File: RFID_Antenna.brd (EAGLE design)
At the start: 25.4 x 43.2 mm, 25 parts, among them J1 U.FL

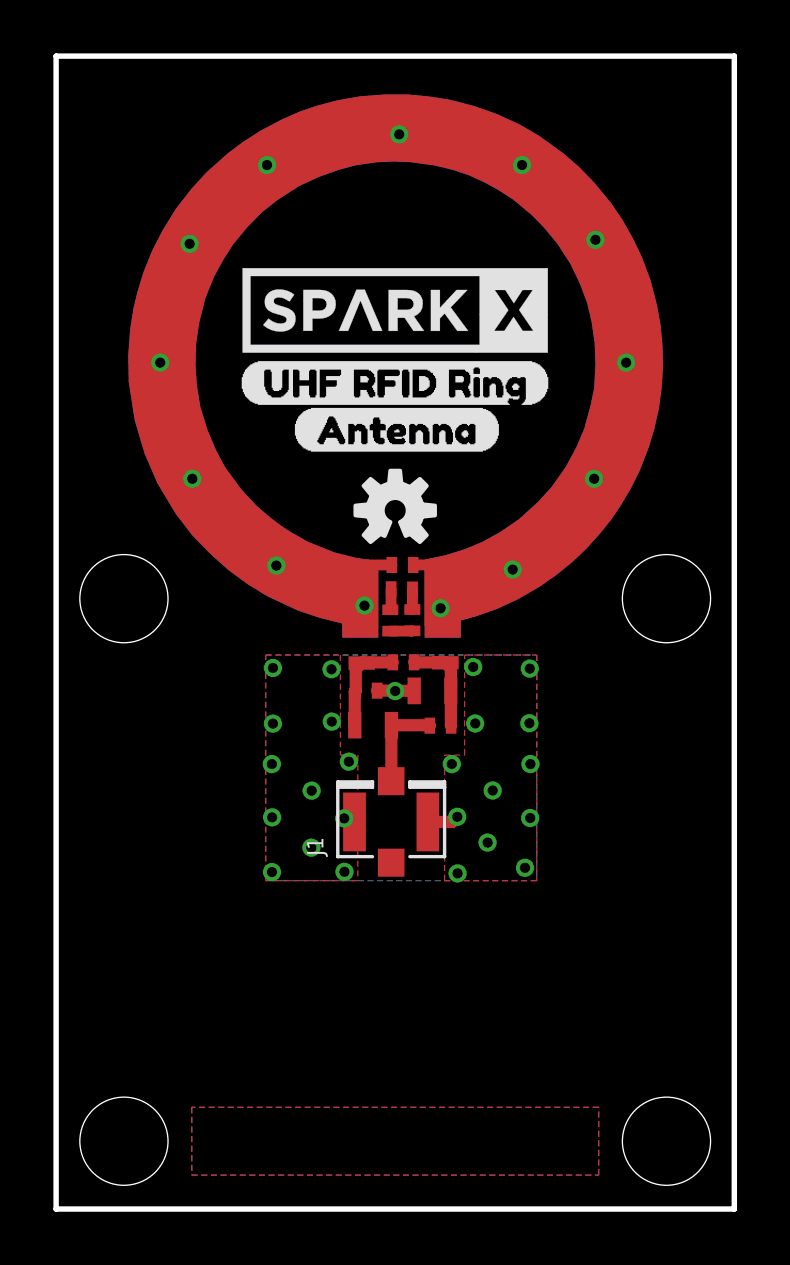
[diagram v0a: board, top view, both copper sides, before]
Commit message: Add production for x02
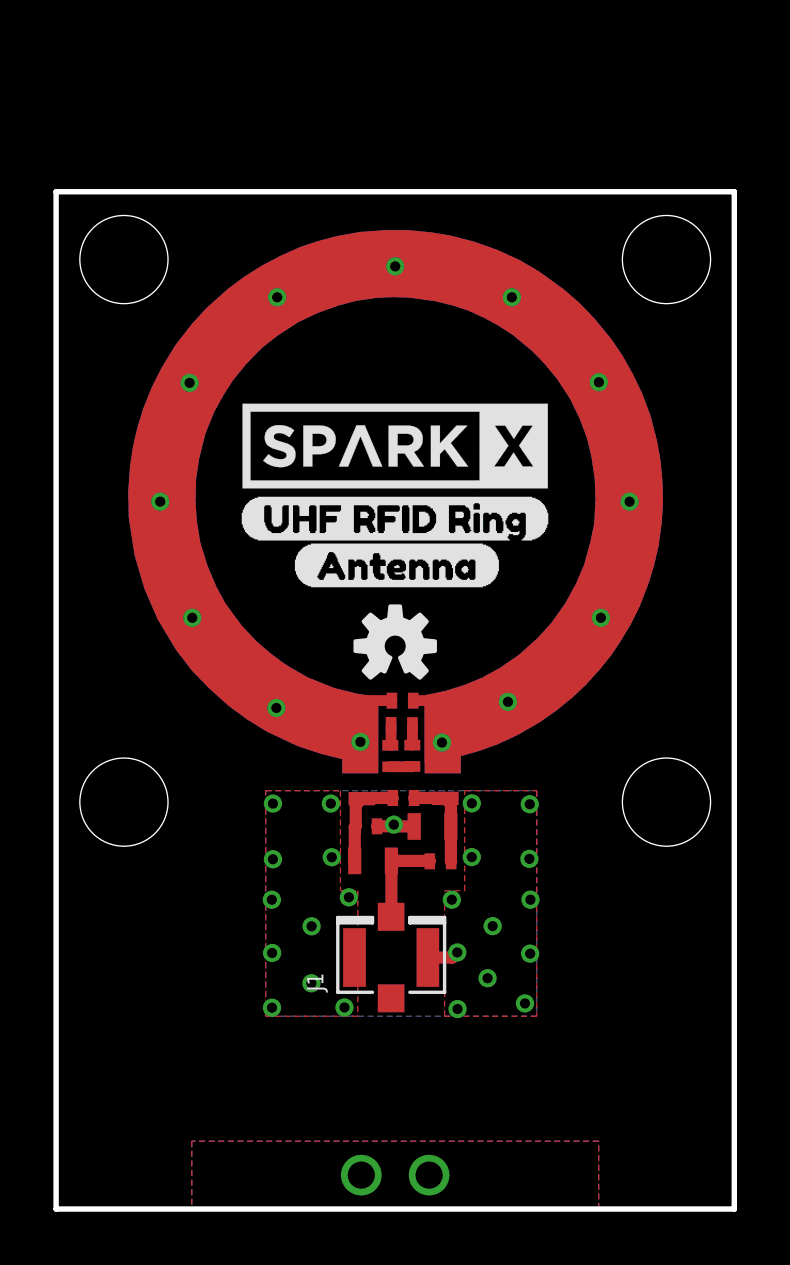
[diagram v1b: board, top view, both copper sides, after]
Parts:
- moved FRAME1 113.1 mm to (-15.2, -66.0)
- moved U$2 66.1 mm to (-34.3, -5.08)
- moved U$11 12.7 mm to (12.7, 25.4)
- moved C2 5.08 mm to (13.7, 18.1)
- moved C3 5.08 mm to (12.5, 17.0)
- moved L3 5.08 mm to (14.6, 16.1)
- moved U$1 5.08 mm to (12.7, 26.7)
- moved U$3 5.08 mm to (12.7, 28.6)
- moved U$4 5.08 mm to (12.7, 28.6)
- moved U$5 5.08 mm to (6.83, 25.9)
- moved U$6 5.08 mm to (18.5, 25.9)
- moved J1 5.08 mm to (12.5, 9.42)
- moved L1 5.08 mm to (13.0, 15.4)
- moved L4 5.08 mm to (14.1, 14.3)
- moved L5 5.08 mm to (11.9, 13.0)
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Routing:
- net GND: track 2.58 -> 2.80 mm, vias 25 -> 24
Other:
- board size 25.4 x 43.2 mm -> 25.4 x 38.1 mm
- board text added: "Owen Lyke"
